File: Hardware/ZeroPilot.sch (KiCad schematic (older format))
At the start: 3 parts, among them J1 CONN_01X04

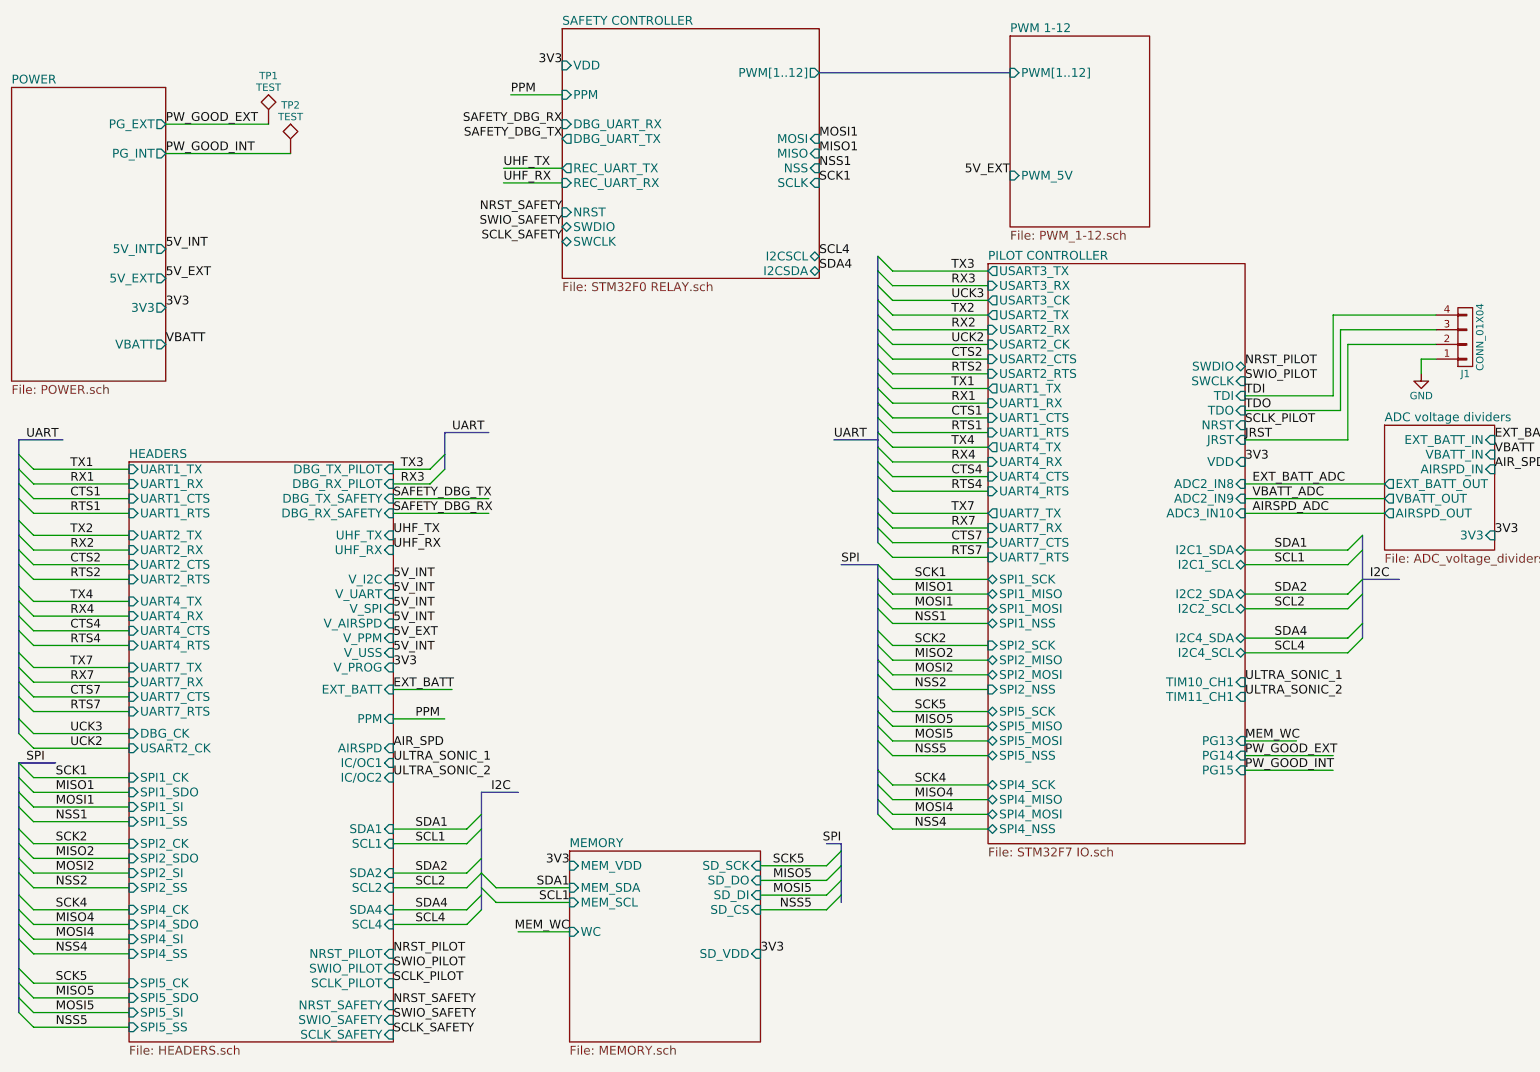
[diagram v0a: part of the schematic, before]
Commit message: Added clock, cleaned up files
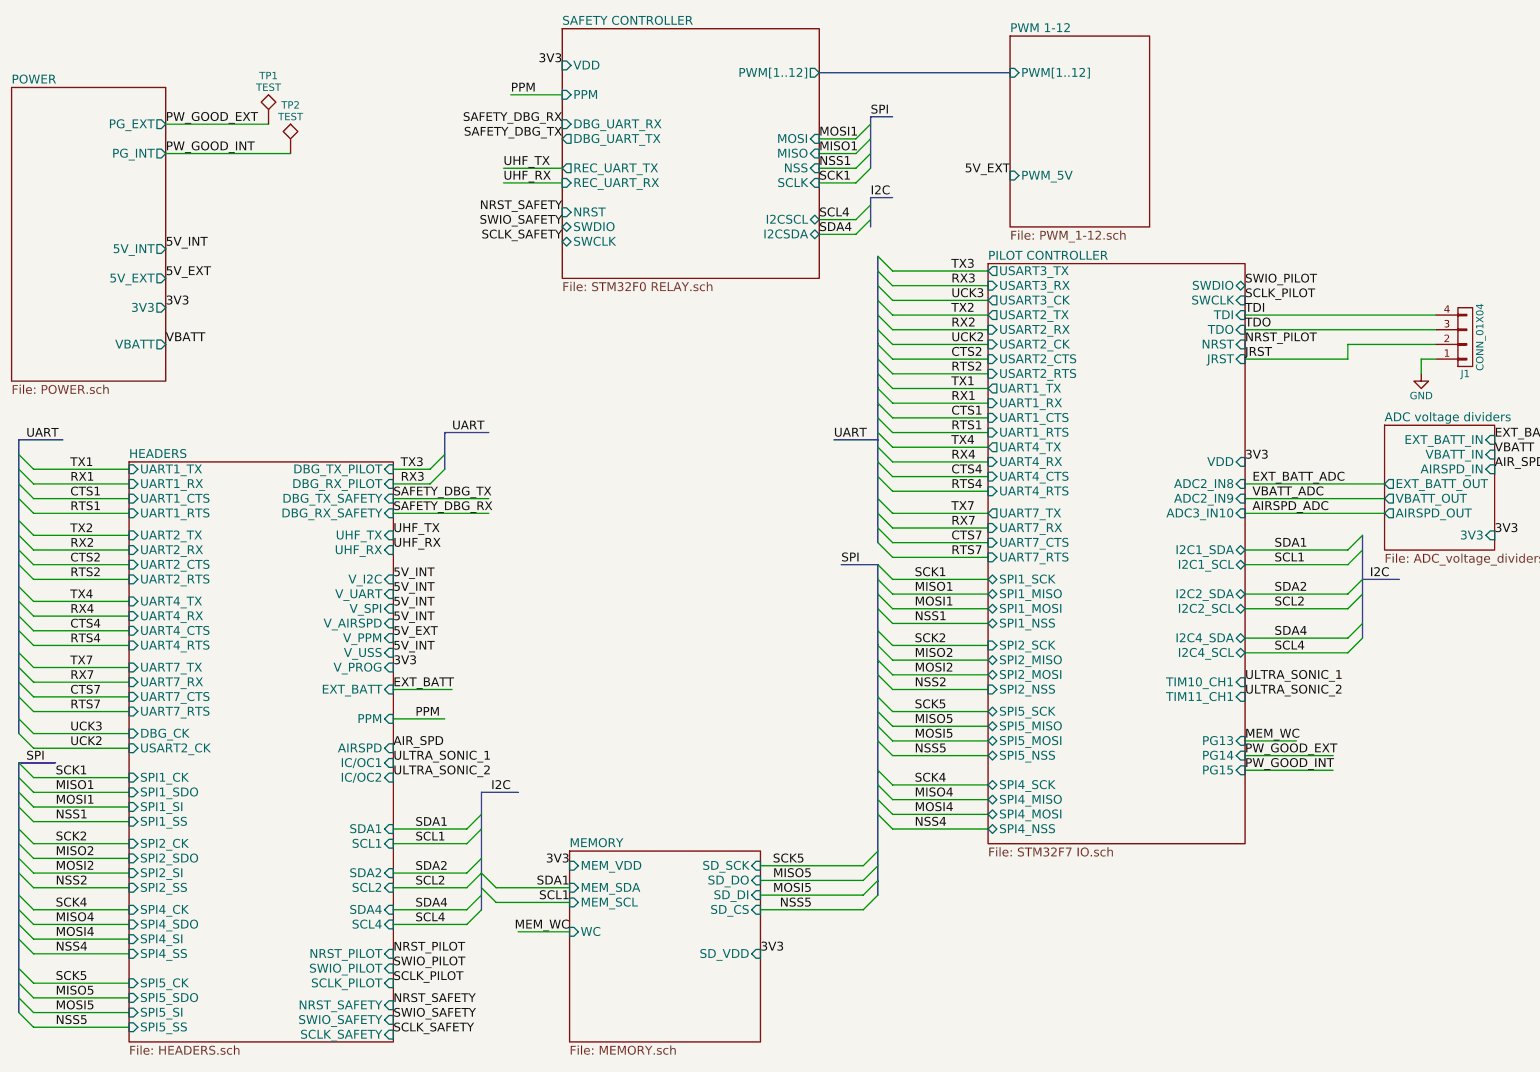
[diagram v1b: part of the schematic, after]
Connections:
- wire segments 117 -> 119
